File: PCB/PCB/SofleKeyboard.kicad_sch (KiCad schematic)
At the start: 117 parts, among them J1 DATA Port, J2 DATA Port, J3 Conn_01x04, J4 , SW1 1u, SW10 1u, SW11 1u, SW12 1u, SW13 1u, SW14 1u, SW15 1u, SW16 1u, SW17 1u, SW18 1u, SW19 1u, SW2 1u, SW20 1u, SW21 1u, SW22 1u, SW23 1u, SW24 1u, SW25 1u, SW26 1u, SW27 1u, SW28 1u, SW29 1u, SW3 1u, SW30 1u, SW31 , SW32 1u, SW33 1u, SW34 1u, SW35 1u, SW36 1u, SW37 1u, SW38 1u, SW39 1u, SW4 1u, SW40 1u, SW41 1u, SW42 1u, SW43 1u, SW44 1u, SW45 1u, SW46 1.5u, SW47 , SW48 , SW5 1u, SW6 1u, SW7 1u, SW8 1u, SW9 1u, U1 Promicro, U2 Blackpill-F4x1

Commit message: cap nhat 11:55 13/06/2022
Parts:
- R1, R2: footprint Resistor_SMD:R_0603_1608Metric -> Library:R_0805_2012Metric_Pad1.20x1.40mm_HandSolder
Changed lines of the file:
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@@
       (effects (font (size 1.27 1.27)) (justify left))
     )
-    (property "Footprint" "Resistor_SMD:R_0603_1608Metric" (id 2) (at 61.722 95.25 90)
+    (property "Footprint" "Library:R_0805_2012Metric_Pad1.20x1.40mm_HandSolder" (id 2) (at 61.722 95.25 90)
       (effects (font (size 1.27 1.27)) hide)
     )
@@
       (effects (font (size 1.27 1.27)) (justify left))
     )
-    (property "Footprint" "Resistor_SMD:R_0603_1608Metric" (id 2) (at 55.372 95.25 90)
+    (property "Footprint" "Library:R_0805_2012Metric_Pad1.20x1.40mm_HandSolder" (id 2) (at 55.372 95.25 90)
       (effects (font (size 1.27 1.27)) hide)
     )
@@
       (reference "#PWR0109") (unit 1) (value "+3.3V") (footprint "")
     )
+    (path "/d5f0102a-ccd2-481d-aac9-a500663069d8/de2ae919-ef2c-4c13-b65e-4e2417e55785"
+      (reference "#PWR0110") (unit 1) (value "+3.3V") (footprint "")
+    )
+    (path "/d5f0102a-ccd2-481d-aac9-a500663069d8/c0a34e97-87d6-47e8-a2c2-8827172c43ef"
+      (reference "#PWR0111") (unit 1) (value "+3.3V") (footprint "")
+    )
+    (path "/d5f0102a-ccd2-481d-aac9-a500663069d8/c4dab5f1-5786-46db-ab7a-1b44fd1dd33c"
+      (reference "#PWR0112") (unit 1) (value "+3.3V") (footprint "")
+    )
+    (path "/d5f0102a-ccd2-481d-aac9-a500663069d8/1a2cbb7d-a12b-4ce2-8cb5-723dbf106184"
+      (reference "#PWR0113") (unit 1) (value "GND") (footprint "")
+    )
+    (path "/d5f0102a-ccd2-481d-aac9-a500663069d8/ea622771-3cf0-4c6c-863e-6326c4f96725"
+      (reference "#PWR0114") (unit 1) (value "+3.3V") (footprint "")
+    )
+    (path "/d5f0102a-ccd2-481d-aac9-a500663069d8/2eec7e7a-4330-4f6e-9016-3a7281b4315e"
+      (reference "#PWR0115") (unit 1) (value "GND") (footprint "")
+    )
+    (path "/d5f0102a-ccd2-481d-aac9-a500663069d8/dc7ffb7f-ab71-4bf8-9657-248abbf0d595"
+      (reference "#PWR0116") (unit 1) (value "+3.3V") (footprint "")
+    )
+    (path "/d5f0102a-ccd2-481d-aac9-a500663069d8/cd0c9c20-e15d-4fe8-86ae-a7aa89b66ad5"
+      (reference "#PWR0117") (unit 1) (value "GND") (footprint "")
+    )
+    (path "/d5f0102a-ccd2-481d-aac9-a500663069d8/239ba5d9-a1e7-472b-9463-5fd60ba27aec"
+      (reference "#PWR0118") (unit 1) (value "+3.3V") (footprint "")
+    )
+    (path "/d5f0102a-ccd2-481d-aac9-a500663069d8/e05ab311-16ee-4afe-afba-54842d71dc7d"
+      (reference "#PWR0119") (unit 1) (value "GND") (footprint "")
+    )
+    (path "/d5f0102a-ccd2-481d-aac9-a500663069d8/2ce8521d-b4f6-41fe-a3f6-e943f0a06d49"
+      (reference "#PWR0120") (unit 1) (value "+3.3V") (footprint "")
+    )
+    (path "/d5f0102a-ccd2-481d-aac9-a500663069d8/85636cb1-c8ea-4762-a108-8c9d6362caf3"
+      (reference "#PWR0121") (unit 1) (value "GND") (footprint "")
+    )
+    (path "/d5f0102a-ccd2-481d-aac9-a500663069d8/5de4fbb2-1b94-40fa-a7eb-5ad36fe8b0cd"
+      (reference "#PWR0122") (unit 1) (value "GND") (footprint "")
+    )
+    (path "/d5f0102a-ccd2-481d-aac9-a500663069d8/bd24c0cc-ba9e-4303-87ac-871ef5acb4de"
+      (reference "#PWR0123") (unit 1) (value "+3.3V") (footprint "")
+    )
+    (path "/d5f0102a-ccd2-481d-aac9-a500663069d8/9e7456c4-7fc3-45aa-88a0-82140af05094"
+      (reference "#PWR0124") (unit 1) (value "GND") (footprint "")
+    )
+    (path "/d5f0102a-ccd2-481d-aac9-a500663069d8/3edb8056-dfbd-4dc3-b4f3-1a443b05e4c3"
+      (reference "#PWR0125") (unit 1) (value "GND") (footprint "")
+    )
+    (path "/d5f0102a-ccd2-481d-aac9-a500663069d8/d5d32a32-b3bf-455c-a349-308eaf785aff"
+      (reference "#PWR0126") (unit 1) (value "GND") (footprint "")
+    )
+    (path "/d5f0102a-ccd2-481d-aac9-a500663069d8/c0a2fe72-5e38-4b73-93ef-62b27577e2dc"
+      (reference "#PWR0127") (unit 1) (value "GND") (footprint "")
+    )
+    (path "/d5f0102a-ccd2-481d-aac9-a500663069d8/623a95d3-92aa-43fc-bfb7-1927169d4600"
+      (reference "#PWR0128") (unit 1) (value "+3.3V") (footprint "")
+    )
+    (path "/d5f0102a-ccd2-481d-aac9-a500663069d8/d0eb2768-bb97-4e38-bc3c-5e38821b161a"
+      (reference "#PWR0129") (unit 1) (value "+3.3V") (footprint "")
+    )
     (path "/d5f0102a-ccd2-481d-aac9-a500663069d8/0d44eaf9-a0c8-43b4-a607-55aa510fbbda"
       (reference "C1") (unit 1) (value "104") (footprint "Capacitor_SMD:C_0603_1608Metric")
@@
       (reference "C10") (unit 1) (value "104") (footprint "Capacitor_SMD:C_0603_1608Metric")
     )
+    (path "/d5f0102a-ccd2-481d-aac9-a500663069d8/f7a08f47-28a3-4664-b73f-efd412909c91"
+      (reference "C11") (unit 1) (value "104") (footprint "Capacitor_SMD:C_0603_1608Metric")
+    )
+    (path "/d5f0102a-ccd2-481d-aac9-a500663069d8/3fc5f0c6-b153-4d2b-a97b-280ebd06937c"
+      (reference "C12") (unit 1) (value "104") (footprint "Capacitor_SMD:C_0603_1608Metric")
+    )
+    (path "/d5f0102a-ccd2-481d-aac9-a500663069d8/3ad3e90c-da30-40da-b83d-347234a4d46b"
+      (reference "C13") (unit 1) (value "104") (footprint "Capacitor_SMD:C_0603_1608Metric")
+    )
+    (path "/d5f0102a-ccd2-481d-aac9-a500663069d8/daa113bb-7151-408c-9a5d-9fc0742a8799"
+      (reference "C14") (unit 1) (value "104") (footprint "Capacitor_SMD:C_0603_1608Metric")
+    )
+    (path "/d5f0102a-ccd2-481d-aac9-a500663069d8/f77e1cf1-10b8-41d1-9804-feb0bc1d2b6c"
+      (reference "C15") (unit 1) (value "104") (footprint "Capacitor_SMD:C_0603_1608Metric")
+    )
+    (path "/d5f0102a-ccd2-481d-aac9-a500663069d8/c8c3ba6e-6f6e-4a97-b351-bbff9b9bdcc2"
+      (reference "C16") (unit 1) (value "104") (footprint "Capacitor_SMD:C_0603_1608Metric")
+    )
+    (path "/d5f0102a-ccd2-481d-aac9-a500663069d8/4d8f03af-088e-4619-bd96-718d9784eab5"
+      (reference "C17") (unit 1) (value "104") (footprint "Capacitor_SMD:C_0603_1608Metric")
+    )
+    (path "/d5f0102a-ccd2-481d-aac9-a500663069d8/f2c834f9-c103-4334-8883-5d3b18f11be6"
+      (reference "C18") (unit 1) (value "104") (footprint "Capacitor_SMD:C_0603_1608Metric")
+    )
+    (path "/d5f0102a-ccd2-481d-aac9-a500663069d8/e1581e33-26a5-41d6-8d99-da00ff6956c5"
+      (reference "C19") (unit 1) (value "104") (footprint "Capacitor_SMD:C_0603_1608Metric")
+    )
+    (path "/d5f0102a-ccd2-481d-aac9-a500663069d8/40c4c9f9-f780-4cff-b616-381fe6ca3a50"
+      (reference "C20") (unit 1) (value "104") (footprint "Capacitor_SMD:C_0603_1608Metric")
+    )
     (path "/91aa030c-cd7a-4bf6-a3e6-bccd5e0d552c"
       (reference "D1") (unit 1) (value "D") (footprint "Library:Diode")
@@
     )
     (path "/633aafcb-e7f5-4f49-b90e-2af365a07e52"
-      (reference "R1") (unit 1) (value "10k") (footprint "Resistor_SMD:R_0603_1608Metric")
+      (reference "R1") (unit 1) (value "10k") (footprint "Library:R_0805_2012Metric_Pad1.20x1.40mm_HandSolder")
     )
     (path "/47bef882-7796-4249-9d91-9e6b1c94b8bb"
-      (reference "R2") (unit 1) (value "10k") (footprint "Resistor_SMD:R_0603_1608Metric")
+      (reference "R2") (unit 1) (value "10k") (footprint "Library:R_0805_2012Metric_Pad1.20x1.40mm_HandSolder")
     )
     (path "/e7dfaf12-5663-403e-b5a3-586865df3607"

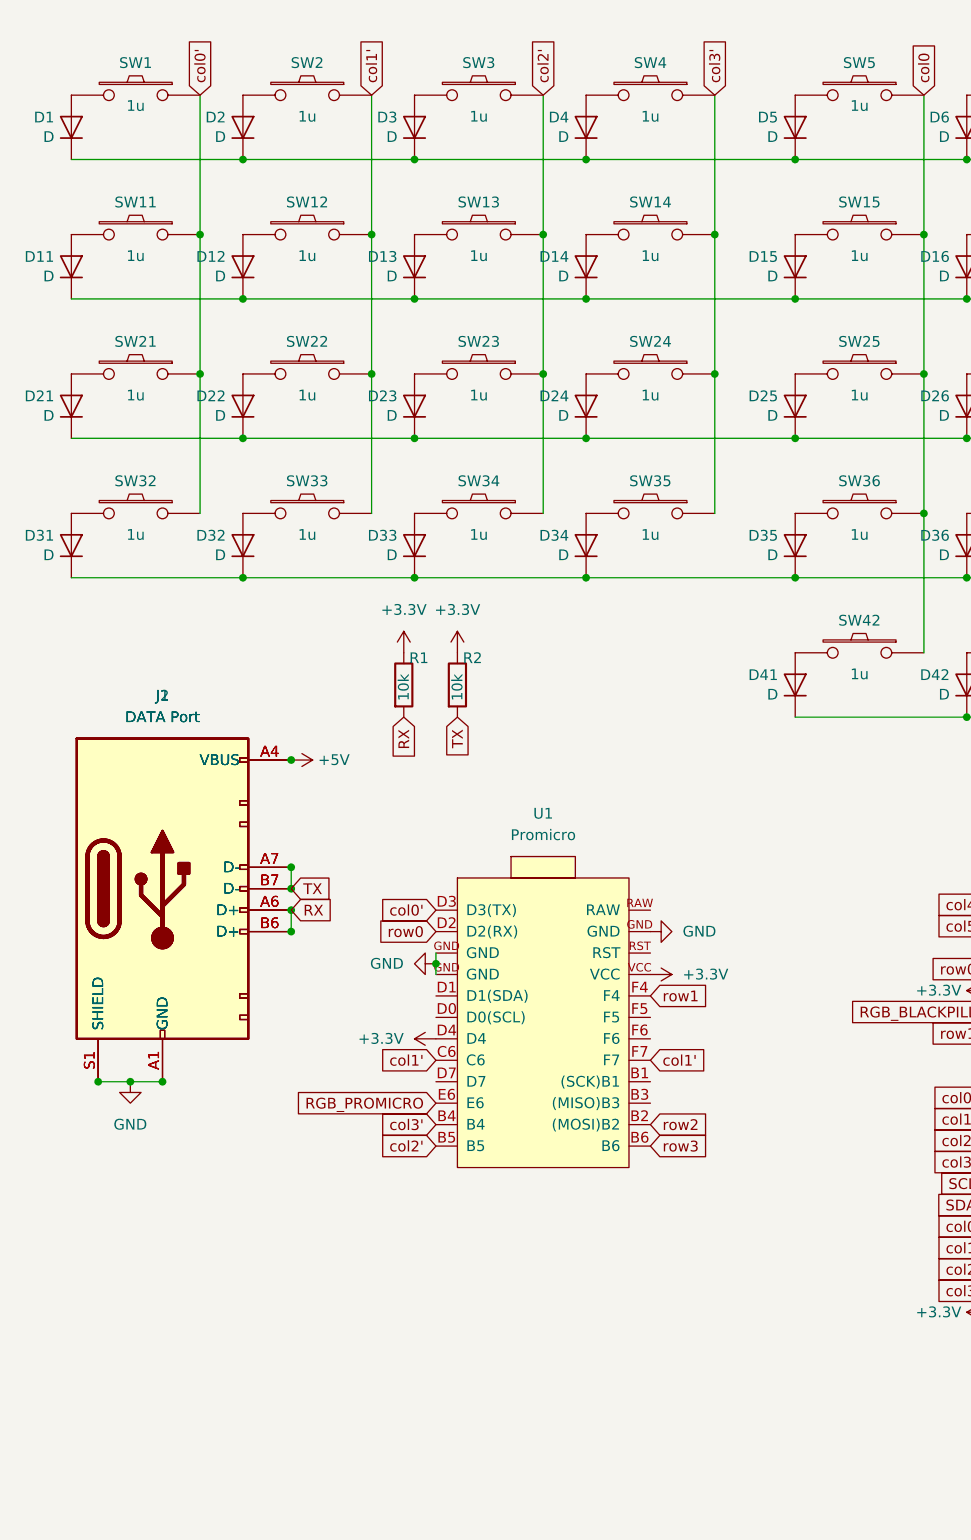
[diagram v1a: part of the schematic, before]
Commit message: 18:29 13/06/2022
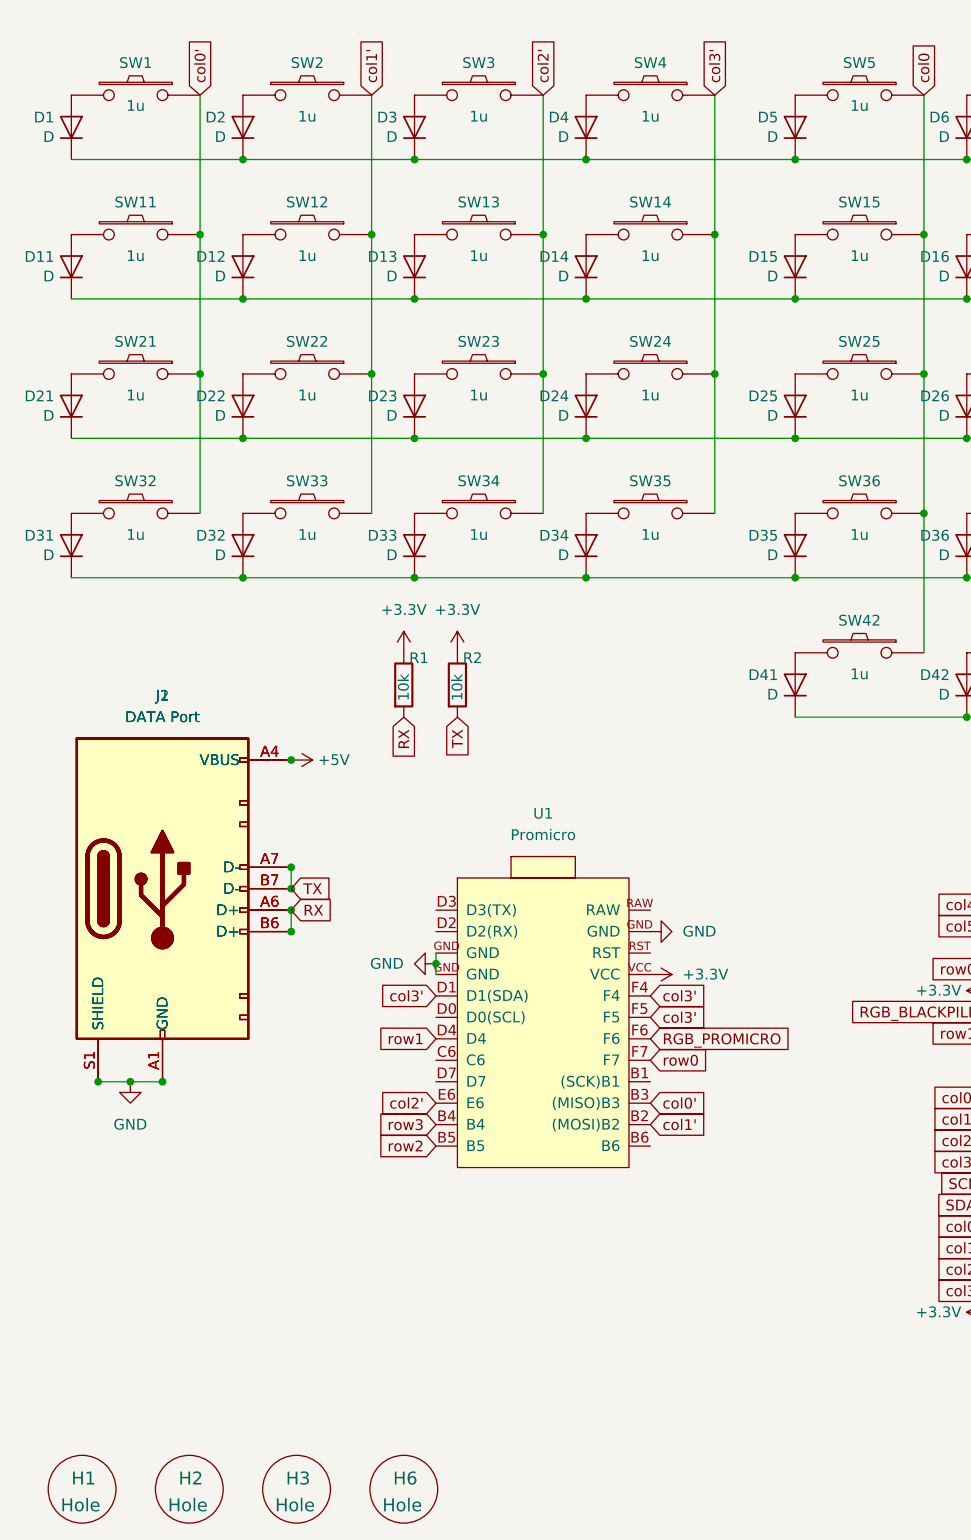
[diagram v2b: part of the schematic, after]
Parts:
- added H1, H2, H3, H6: Hole, Library:Cut_hole, symbol keebio:Hole
- SW11, SW12: footprint Library:SW-HS-Flip-1u -> Library:SW-HS_flip-1u
- SW13, SW14: footprint Library:SW-HS_flip-1u -> Library:SW-HS-Flip-1u
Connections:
- net +3V3: no longer U1.D4
- net RGB_PROMICRO: now also U1.F6; no longer U1.E6
- net col0': now also U1.B3 ((MISO)B3); no longer U1.D3 (D3(TX))
- net col1': now also SW2.2, U1.B2 ((MOSI)B2); no longer SW2.1, U1.C6, U1.F7
- net col2': now also U1.E6; no longer U1.B5
- net col3': now also U1.D1 (D1(SDA)), U1.F4, U1.F5; no longer U1.B4
- net row0: now also U1.F7; no longer U1.D2 (D2(RX))
- net row1: now also U1.D4; no longer U1.F4
- net row2: now also U1.B5; no longer U1.B2 ((MOSI)B2)
- net row3: now also U1.B4; no longer U1.B6
- net at D2.2 (A): now also SW2.1; no longer SW2.2
